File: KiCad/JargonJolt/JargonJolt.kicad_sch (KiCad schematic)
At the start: 0 parts

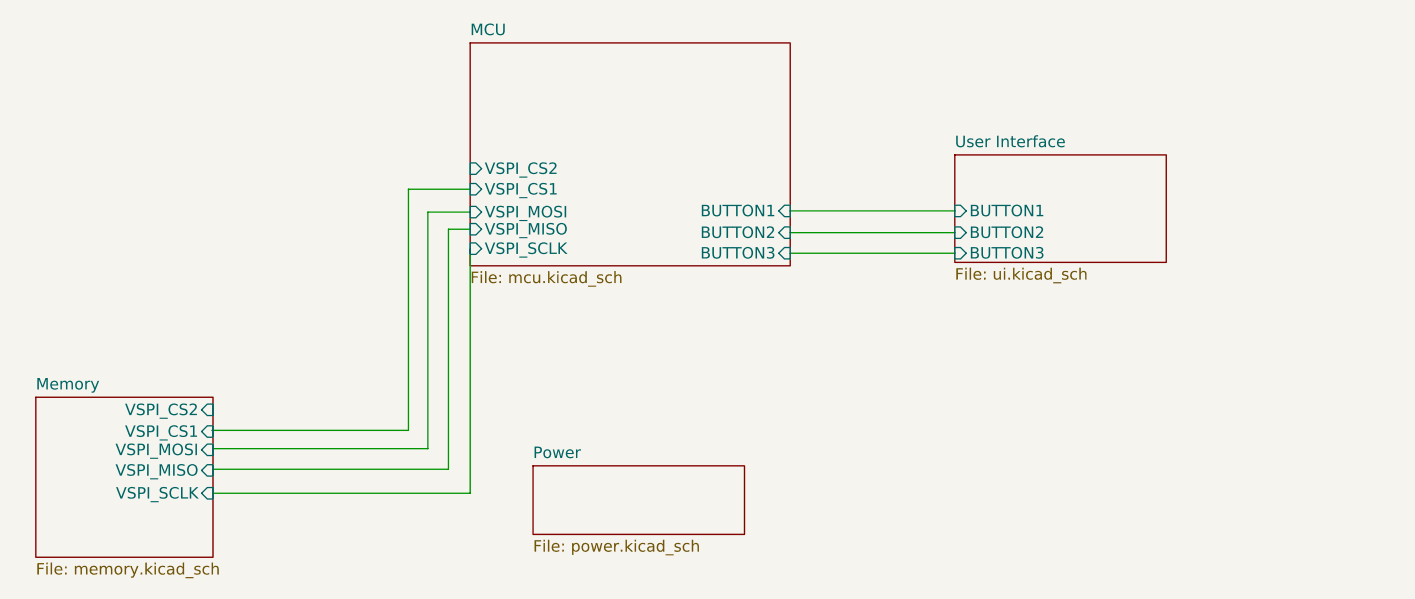
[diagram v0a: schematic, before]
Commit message: worked on schematic
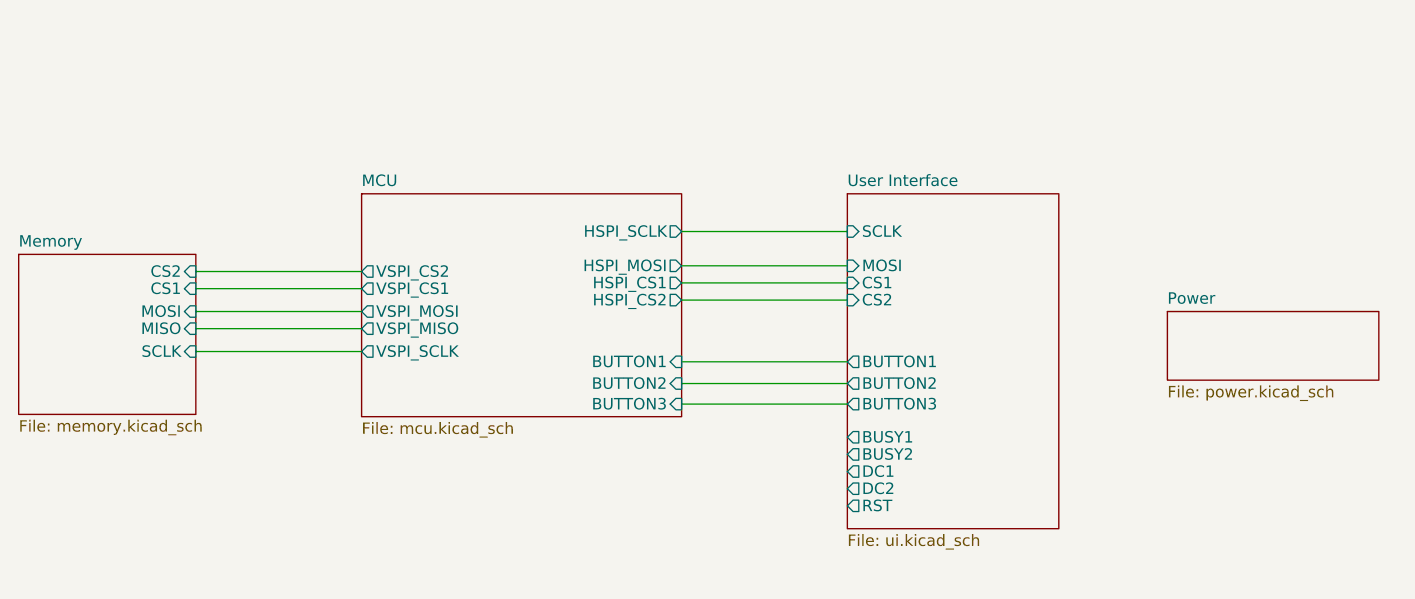
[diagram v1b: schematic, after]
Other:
- sheet MCU ports: added HSPI_CS1, HSPI_CS2, HSPI_MOSI, HSPI_SCLK; removed none
- sheet Memory ports: added CS1, CS2, MISO, MOSI, SCLK; removed VSPI_CS1, VSPI_CS2, VSPI_MISO, VSPI_MOSI, VSPI_SCLK
- sheet User Interface ports: added BUSY1, BUSY2, CS1, CS2, DC1, DC2, MOSI, RST, SCLK; removed none
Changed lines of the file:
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@@
 (kicad_sch (version 20230121) (generator eeschema)
   (paper "A4")
-  (wire (pts (xy 107.061 86.106) (xy 111.76 86.106))
+  (wire (pts (xy 135.255 107.442) (xy 153.67 107.442))
     (stroke (width 0) (type default))
   )
-  (wire (pts (xy 83.312 117.348) (xy 111.76 117.348))
+  (wire (pts (xy 81.28 101.6) (xy 99.695 101.6))
     (stroke (width 0) (type default))
   )
-  (wire (pts (xy 83.185 114.681) (xy 109.347 114.681))
+  (wire (pts (xy 135.255 93.98) (xy 153.67 93.98))
     (stroke (width 0) (type default))
   )
-  (wire (pts (xy 83.185 112.395) (xy 107.061 112.395))
+  (wire (pts (xy 81.28 94.615) (xy 99.695 94.615))
     (stroke (width 0) (type default))
   )
-  (wire (pts (xy 147.32 90.678) (xy 165.608 90.678))
+  (wire (pts (xy 135.255 102.743) (xy 153.67 102.743))
     (stroke (width 0) (type default))
   )
-  (wire (pts (xy 109.347 114.681) (xy 109.347 88.011))
+  (wire (pts (xy 81.28 97.155) (xy 99.695 97.155))
     (stroke (width 0) (type default))
   )
-  (wire (pts (xy 147.32 85.979) (xy 165.608 85.979))
+  (wire (pts (xy 135.255 92.075) (xy 153.67 92.075))
     (stroke (width 0) (type default))
   )
-  (wire (pts (xy 107.061 112.395) (xy 107.061 86.106))
+  (wire (pts (xy 81.28 92.71) (xy 99.695 92.71))
     (stroke (width 0) (type default))
   )
-  (wire (pts (xy 104.902 83.566) (xy 111.76 83.566))
+  (wire (pts (xy 135.255 95.885) (xy 153.67 95.885))
     (stroke (width 0) (type default))
   )
-  (wire (pts (xy 147.32 88.392) (xy 165.608 88.392))
+  (wire (pts (xy 81.28 99.06) (xy 99.695 99.06))
     (stroke (width 0) (type default))
   )
-  (wire (pts (xy 83.058 110.363) (xy 104.902 110.363))
+  (wire (pts (xy 135.255 105.156) (xy 153.67 105.156))
     (stroke (width 0) (type default))
   )
-  (wire (pts (xy 109.347 88.011) (xy 111.76 88.011))
+  (wire (pts (xy 135.255 88.265) (xy 153.67 88.265))
     (stroke (width 0) (type default))
   )
-  (wire (pts (xy 111.76 117.348) (xy 111.76 90.17))
-    (stroke (width 0) (type default))
-  )
-  (wire (pts (xy 104.902 110.363) (xy 104.902 83.566))
-    (stroke (width 0) (type default))
-  )
-  (sheet (at 165.608 79.756) (size 23.495 11.938) (fields_autoplaced)
+  (sheet (at 153.67 84.074) (size 23.495 37.211) (fields_autoplaced)
     (stroke (width 0.1524) (type solid))
     (fill (color 200 255 102 1.0000))
-    (property "Sheetname" "User Interface" (at 165.608 79.0444 0)
+    (property "Sheetname" "User Interface" (at 153.67 83.3624 0)
       (effects (font (size 1.27 1.27)) (justify left bottom))
     )
-    (property "Sheetfile" "ui.kicad_sch" (at 165.608 92.2786 0)
+    (property "Sheetfile" "ui.kicad_sch" (at 153.67 121.8696 0)
       (effects (font (size 1.27 1.27)) (justify left top))
     )
-    (pin "BUTTON1" input (at 165.608 85.979 180)
+    (pin "BUTTON1" output (at 153.67 102.743 180)
       (effects (font (size 1.27 1.27)) (justify left))
     )
-    (pin "BUTTON2" input (at 165.608 88.392 180)
+    (pin "BUTTON2" output (at 153.67 105.156 180)
       (effects (font (size 1.27 1.27)) (justify left))
     )
-    (pin "BUTTON3" input (at 165.608 90.678 180)
+    (pin "BUTTON3" output (at 153.67 107.442 180)
+      (effects (font (size 1.27 1.27)) (justify left))
+    )
+    (pin "SCLK" input (at 153.67 88.265 180)
+      (effects (font (size 1.27 1.27)) (justify left))
+    )
+    (pin "MOSI" input (at 153.67 92.075 180)
+      (effects (font (size 1.27 1.27)) (justify left))
+    )
+    (pin "CS1" input (at 153.67 93.98 180)
+      (effects (font (size 1.27 1.27)) (justify left))
+    )
+    (pin "CS2" input (at 153.67 95.885 180)
+      (effects (font (size 1.27 1.27)) (justify left))
+    )
+    (pin "BUSY1" output (at 153.67 111.125 180)
+      (effects (font (size 1.27 1.27)) (justify left))
+    )
+    (pin "DC2" output (at 153.67 116.84 180)
+      (effects (font (size 1.27 1.27)) (justify left))
+    )
+    (pin "BUSY2" output (at 153.67 113.03 180)
+      (effects (font (size 1.27 1.27)) (justify left))
+    )
+    (pin "DC1" output (at 153.67 114.935 180)
+      (effects (font (size 1.27 1.27)) (justify left))
+    )
+    (pin "RST" output (at 153.67 118.745 180)
       (effects (font (size 1.27 1.27)) (justify left))
     )
@@
     )
   )
-  (sheet (at 63.5 106.68) (size 19.685 17.78) (fields_autoplaced)
+  (sheet (at 61.595 90.805) (size 19.685 17.78) (fields_autoplaced)
     (stroke (width 0.1524) (type solid))
     (fill (color 113 64 255 1.0000))
-    (property "Sheetname" "Memory" (at 63.5 105.9684 0)
+    (property "Sheetname" "Memory" (at 61.595 90.0934 0)
       (effects (font (size 1.27 1.27)) (justify left bottom))
     )
-    (property "Sheetfile" "memory.kicad_sch" (at 63.5 125.0446 0)
+    (property "Sheetfile" "memory.kicad_sch" (at 61.595 109.1696 0)
       (effects (font (size 1.27 1.27)) (justify left top))
     )
-    (pin "VSPI_CS1" input (at 83.185 110.49 0)
+    (pin "MISO" input (at 81.28 99.06 0)
       (effects (font (size 1.27 1.27)) (justify right))
     )
-    (pin "VSPI_MOSI" input (at 83.185 112.522 0)
+    (pin "CS1" input (at 81.28 94.615 0)
       (effects (font (size 1.27 1.27)) (justify right))
     )
-    (pin "VSPI_MISO" input (at 83.185 114.808 0)
+    (pin "CS2" input (at 81.28 92.71 0)
       (effects (font (size 1.27 1.27)) (justify right))
     )
-    (pin "VSPI_CS2" input (at 83.185 108.077 0)
+    (pin "MOSI" input (at 81.28 97.155 0)
       (effects (font (size 1.27 1.27)) (justify right))
     )
-    (pin "VSPI_SCLK" input (at 83.185 117.348 0)
+    (pin "SCLK" input (at 81.28 101.6 0)
       (effects (font (size 1.27 1.27)) (justify right))
     )
@@
     )
   )
-  (sheet (at 118.745 114.3) (size 23.495 7.62) (fields_autoplaced)
+  (sheet (at 189.23 97.155) (size 23.495 7.62) (fields_autoplaced)
     (stroke (width 0.1524) (type solid))
     (fill (color 255 94 97 1.0000))
-    (property "Sheetname" "Power" (at 118.745 113.5884 0)
+    (property "Sheetname" "Power" (at 189.23 96.4434 0)
       (effects (font (size 1.27 1.27)) (justify left bottom))
     )
-    (property "Sheetfile" "power.kicad_sch" (at 118.745 122.5046 0)
+    (property "Sheetfile" "power.kicad_sch" (at 189.23 105.3596 0)
       (effects (font (size 1.27 1.27)) (justify left top))
     )
@@
     )
   )
-  (sheet (at 111.76 67.31) (size 35.56 24.765) (fields_autoplaced)
+  (sheet (at 99.695 84.074) (size 35.56 24.765) (fields_autoplaced)
     (stroke (width 0.1524) (type solid))
     (fill (color 91 138 255 1.0000))
-    (property "Sheetname" "MCU" (at 111.76 66.5984 0)
+    (property "Sheetname" "MCU" (at 99.695 83.3624 0)
       (effects (font (size 1.27 1.27)) (justify left bottom))
     )
-    (property "Sheetfile" "mcu.kicad_sch" (at 111.76 92.6596 0)
+    (property "Sheetfile" "mcu.kicad_sch" (at 99.695 109.4236 0)
       (effects (font (size 1.27 1.27)) (justify left top))
     )
-    (pin "BUTTON1" input (at 147.32 85.979 0)
+    (pin "BUTTON1" input (at 135.255 102.743 0)
       (effects (font (size 1.27 1.27)) (justify right))
     )
-    (pin "BUTTON2" input (at 147.32 88.392 0)
+    (pin "BUTTON2" input (at 135.255 105.156 0)
       (effects (font (size 1.27 1.27)) (justify right))
     )
-    (pin "VSPI_MOSI" input (at 111.76 86.106 180)
+    (pin "VSPI_MOSI" output (at 99.695 97.155 180)
       (effects (font (size 1.27 1.27)) (justify left))
     )
-    (pin "VSPI_SCLK" input (at 111.76 90.17 180)
+    (pin "VSPI_SCLK" output (at 99.695 101.6 180)
       (effects (font (size 1.27 1.27)) (justify left))
     )
-    (pin "VSPI_MISO" input (at 111.76 88.011 180)
+    (pin "VSPI_MISO" output (at 99.695 99.06 180)
       (effects (font (size 1.27 1.27)) (justify left))
     )
-    (pin "VSPI_CS1" input (at 111.76 83.566 180)
+    (pin "VSPI_CS1" output (at 99.695 94.615 180)
       (effects (font (size 1.27 1.27)) (justify left))
     )
-    (pin "VSPI_CS2" input (at 111.76 81.28 180)
+    (pin "VSPI_CS2" output (at 99.695 92.71 180)
       (effects (font (size 1.27 1.27)) (justify left))
     )
-    (pin "BUTTON3" input (at 147.32 90.678 0)
+    (pin "BUTTON3" input (at 135.255 107.442 0)
       (effects (font (size 1.27 1.27)) (justify right))
     )
+    (pin "HSPI_SCLK" output (at 135.255 88.265 0)
+      (effects (font (size 1.27 1.27)) (justify right))
+    )
+    (pin "HSPI_MOSI" output (at 135.255 92.075 0)
+      (effects (font (size 1.27 1.27)) (justify right))
+    )
+    (pin "HSPI_CS1" output (at 135.255 93.98 0)
+      (effects (font (size 1.27 1.27)) (justify right))
+    )
+    (pin "HSPI_CS2" output (at 135.255 95.885 0)
+      (effects (font (size 1.27 1.27)) (justify right))
+    )
